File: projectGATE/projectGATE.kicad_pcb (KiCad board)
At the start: 2 copper layers, 126 x 63 mm, 22 parts, among them J1 TB009-508-02BE, J2 TB009-508-03BE, J3 TB009-508-03BE, K1 SRD-05VDC-SL-C, K2 SRD-05VDC-SL-C, Q1 BC547, Q2 BC547, U1 ESP32-DEVKITC, U2 PC817, U3 PC817, U4 LM7805_TO220

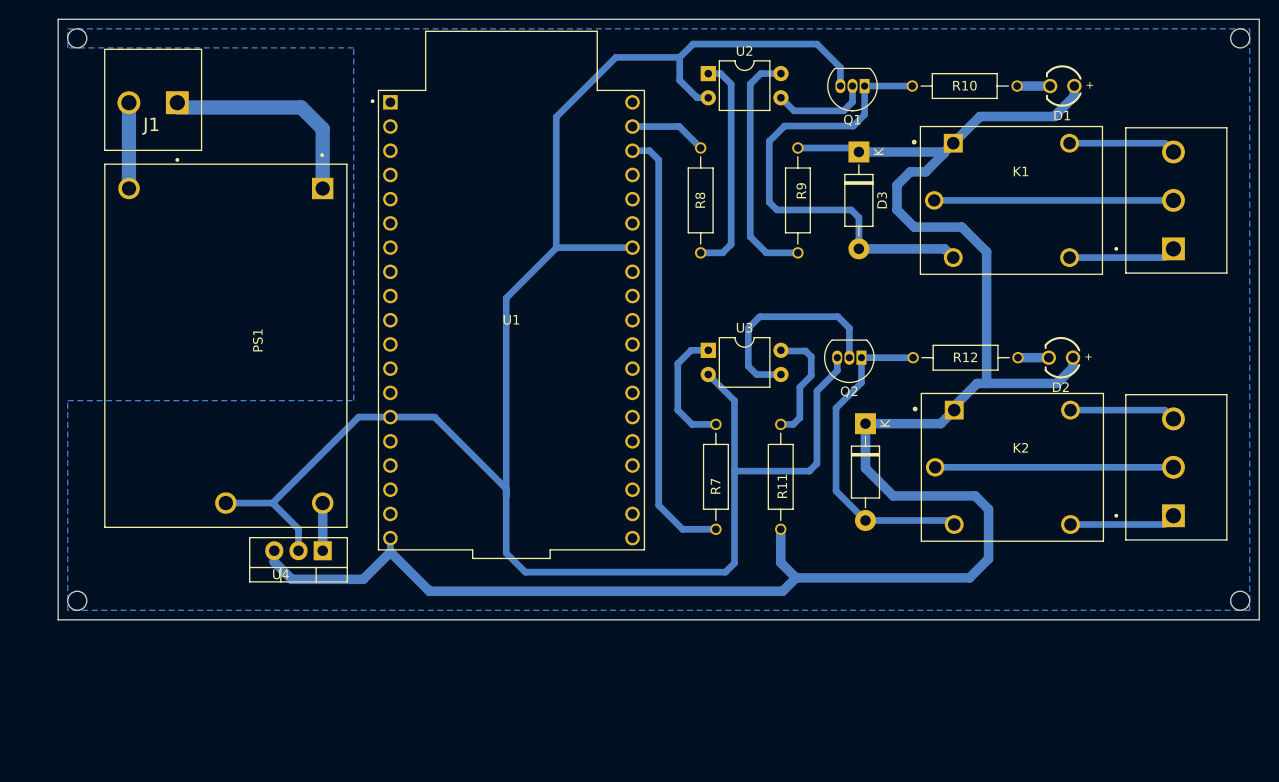
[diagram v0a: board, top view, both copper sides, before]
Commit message: fixx
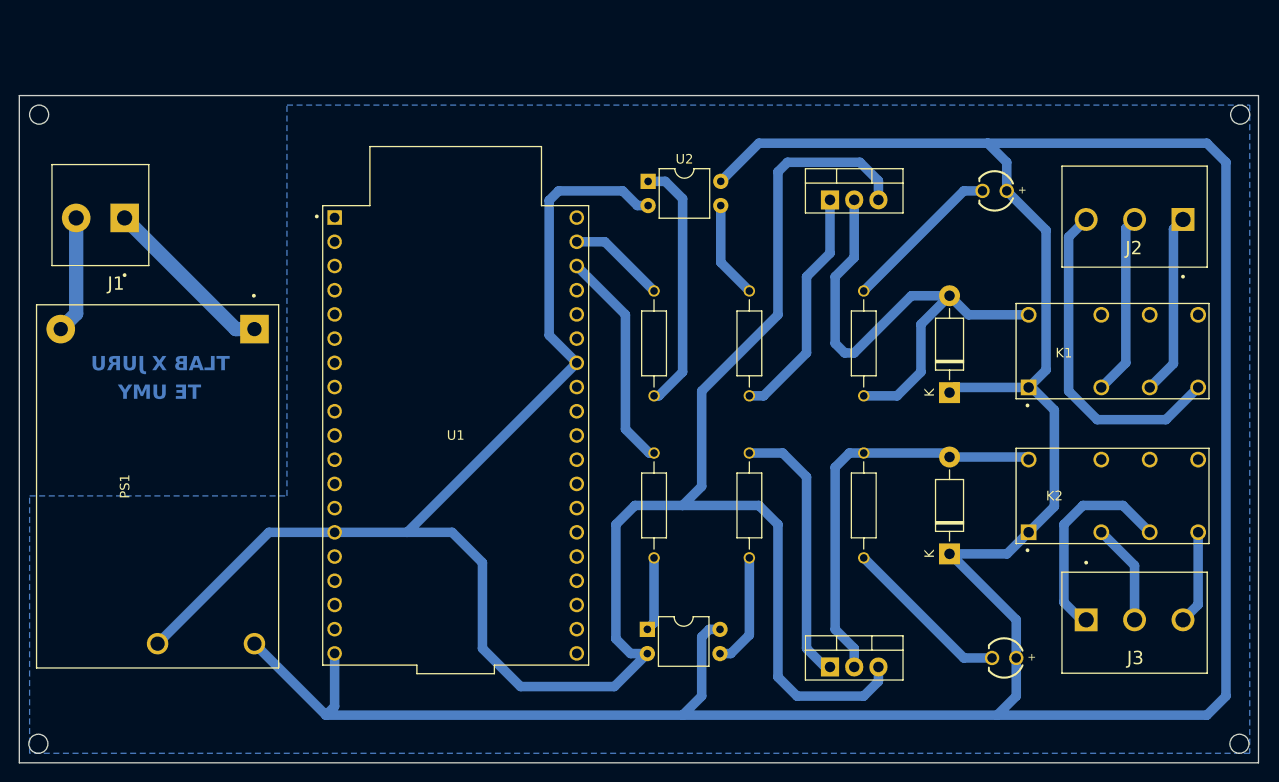
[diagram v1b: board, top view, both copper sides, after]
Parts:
- removed Q1: BC547, Package_TO_SOT_THT:TO-92_Inline
- removed U4: LM7805_TO220, Package_TO_SOT_THT:TO-220-3_Vertical
- added Q3: TIP41, Package_TO_SOT_THT:TO-220-3_Vertical, F.Cu at (170.0, 86.9)
- D1, D2: value WL-TMRC_3MM -> LED 3MM
- K1, K2: value SRD-05VDC-SL-C -> 8-1393792-5; footprint SRD-05VDC-SL-C:RELAY_SRD-05VDC-SL-C -> 8-1393792-5:RELAY_8-1393792-5
- Q2: value BC547 -> TIP41; footprint Package_TO_SOT_THT:TO-92_Inline -> Package_TO_SOT_THT:TO-220-3_Vertical
- R10, R12: value MFR-25FBF52-1K -> 330R
- R11, R9: value MFR-25FBF52-1K -> 2K2
- R7, R8: value MFR-25FBF52-1K -> 220R
- moved Q2 32.6 mm to (170.0, 135.9), turned to 0 degrees
- moved D2 32.1 mm to (188.2, 135.0)
- moved U3 30.0 mm to (150.8, 132.0)
- moved R10 29.0 mm to (173.5, 102.0), turned to -90 degrees
- moved D3 27.0 mm to (182.5, 107.2), turned to 90 degrees
- moved K1 19.0 mm to (199.6, 102.8)
- moved R12 18.8 mm to (173.5, 119.0), turned to 90 degrees
- moved PS1 16.4 mm to (99.4, 117.0)
- moved D4 16.3 mm to (182.5, 124.1), turned to 90 degrees
- moved R9 15.8 mm to (161.5, 102.0), turned to -90 degrees
- moved R8 15.8 mm to (151.5, 102.0)
- moved J3 14.3 mm to (196.8, 131.0), turned to 0 degrees
- moved U1 13.4 mm to (130.7, 111.7)
- moved J1 13.3 mm to (96.0, 88.8)
- moved D1 13.1 mm to (187.2, 86.0)
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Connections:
- PS1 pad 4: Net-(PS1-+VO) -> 5V
- Q2 pad 1: Net-(D4-A) -> Net-(Q2-B)
- Q2 pad 2: Net-(Q2-B) -> Net-(D4-A)
- R11 pad 2: 5V -> Net-(Q2-B)
- R9 pad 2: 5V -> Net-(Q3-B)
- U2 pad 3: Net-(Q1-B) -> Net-(R9-Pad1)
- U2 pad 4: Net-(R9-Pad1) -> 5V
- U3 pad 3: Net-(Q2-B) -> Net-(R11-Pad1)
- U3 pad 4: Net-(R11-Pad1) -> 5V
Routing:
- net 5V: track 205.2 -> 320.5 mm
- net GND: track 208.3 -> 241.5 mm
- net Net-(Q3-B): track 0.00 -> 25.3 mm
- net Net-(J2-Pad3): track 11.3 -> 35.2 mm
- net Net-(U1-IO22): track 46.4 -> 23.3 mm
- net Net-(R9-Pad1): track 25.4 -> 10.2 mm
- net Net-(D2-Pad2): track 3.23 -> 17.8 mm
- net Net-(J3-Pad2): track 25.0 -> 10.6 mm
- net Net-(D1-Pad2): track 3.46 -> 16.8 mm
- net Net-(J3-Pad1): track 11.2 -> 21.8 mm
- net Net-(Q1-B): track 10.1 -> 0.00 mm
- net Net-(D4-A): track 35.0 -> 43.0 mm
- net Net-(J2-Pad1): track 11.3 -> 19.1 mm
- net Net-(D3-A): track 49.2 -> 56.2 mm
- net Net-(J2-Pad2): track 25.1 -> 19.1 mm
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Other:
- board size 126 x 63 mm -> 130 x 70 mm
- board text added: "TE UMY"
- board text added: "TLAB X JURU"
